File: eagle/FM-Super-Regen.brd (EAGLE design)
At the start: 41.9 x 21.6 mm, 15 parts, among them Q1 BF245B

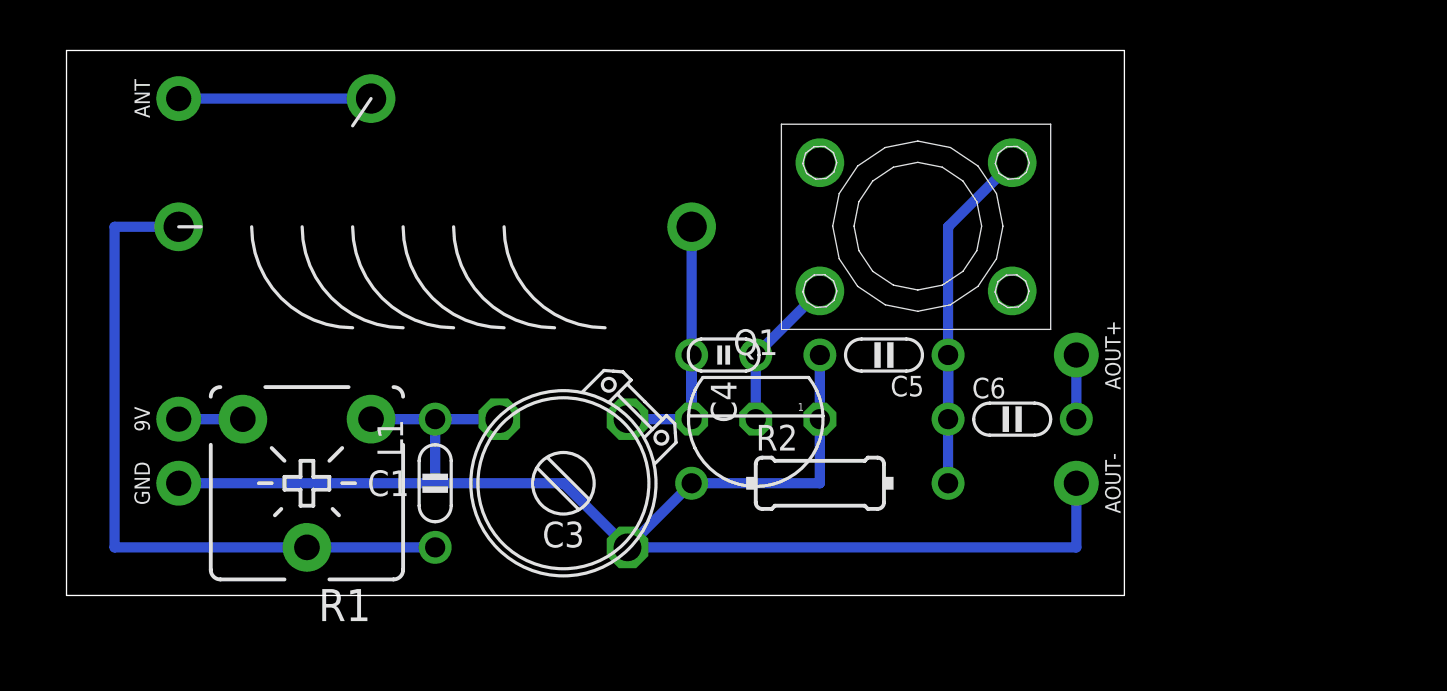
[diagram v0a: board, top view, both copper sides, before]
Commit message: ...
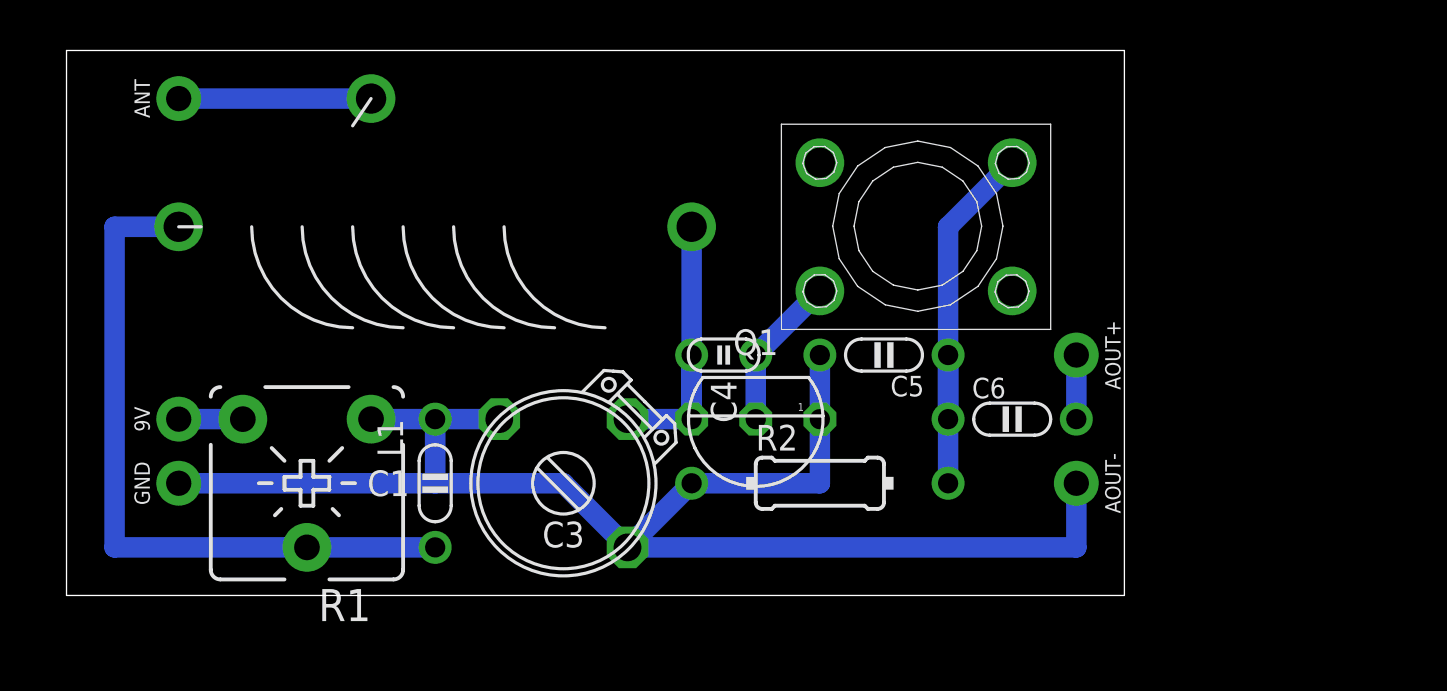
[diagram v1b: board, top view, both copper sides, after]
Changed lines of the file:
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@@
 <?xml version="1.0" encoding="utf-8"?>
 <!DOCTYPE eagle SYSTEM "eagle.dtd">
-<eagle version="7.7.0">
+<eagle version="7.6.0">
 <drawing>
 <settings>
@@
 <contactref element="AOUT-" pad="1"/>
 <contactref element="GND" pad="1"/>
-<wire x1="30.48" y1="7.62" x2="30.48" y2="5.08" width="0.4064" layer="16"/>
-<wire x1="12.7" y1="7.62" x2="15.24" y2="7.62" width="0.4064" layer="16"/>
-<wire x1="5.08" y1="5.08" x2="15.24" y2="5.08" width="0.4064" layer="16"/>
-<wire x1="15.24" y1="5.08" x2="20.32" y2="5.08" width="0.4064" layer="16"/>
-<wire x1="20.32" y1="5.08" x2="22.86" y2="2.54" width="0.4064" layer="16"/>
-<wire x1="17.78" y1="7.62" x2="15.24" y2="7.62" width="0.4064" layer="16"/>
-<wire x1="15.24" y1="7.62" x2="15.24" y2="5.08" width="0.4064" layer="16"/>
-<wire x1="40.64" y1="5.08" x2="40.64" y2="2.54" width="0.4064" layer="16"/>
-<wire x1="40.64" y1="2.54" x2="22.86" y2="2.54" width="0.4064" layer="16"/>
-<wire x1="22.86" y1="2.54" x2="25.4" y2="5.08" width="0.4064" layer="16"/>
-<wire x1="25.4" y1="5.08" x2="30.48" y2="5.08" width="0.4064" layer="16"/>
-<wire x1="30.48" y1="7.62" x2="30.48" y2="10.16" width="0.4064" layer="16"/>
+<wire x1="30.48" y1="7.62" x2="30.48" y2="5.08" width="0.8128" layer="16"/>
+<wire x1="12.7" y1="7.62" x2="15.24" y2="7.62" width="0.8128" layer="16"/>
+<wire x1="5.08" y1="5.08" x2="15.24" y2="5.08" width="0.8128" layer="16"/>
+<wire x1="15.24" y1="5.08" x2="20.32" y2="5.08" width="0.8128" layer="16"/>
+<wire x1="20.32" y1="5.08" x2="22.86" y2="2.54" width="0.8128" layer="16"/>
+<wire x1="17.78" y1="7.62" x2="15.24" y2="7.62" width="0.8128" layer="16"/>
+<wire x1="15.24" y1="7.62" x2="15.24" y2="5.08" width="0.8128" layer="16"/>
+<wire x1="40.64" y1="5.08" x2="40.64" y2="2.54" width="0.8128" layer="16"/>
+<wire x1="40.64" y1="2.54" x2="22.86" y2="2.54" width="0.8128" layer="16"/>
+<wire x1="22.86" y1="2.54" x2="25.4" y2="5.08" width="0.8128" layer="16"/>
+<wire x1="25.4" y1="5.08" x2="30.48" y2="5.08" width="0.8128" layer="16"/>
+<wire x1="30.48" y1="7.62" x2="30.48" y2="10.16" width="0.8128" layer="16"/>
 </signal>
 <signal name="N$2">
@@
 <contactref element="C4" pad="1"/>
 <contactref element="C3" pad="2"/>
-<wire x1="25.4" y1="15.24" x2="25.4" y2="7.62" width="0.4064" layer="16"/>
-<wire x1="25.4" y1="10.16" x2="25.4" y2="7.62" width="0.4064" layer="16"/>
-<wire x1="25.4" y1="7.62" x2="22.86" y2="7.62" width="0.4064" layer="16"/>
+<wire x1="25.4" y1="15.24" x2="25.4" y2="7.62" width="0.8128" layer="16"/>
+<wire x1="25.4" y1="10.16" x2="25.4" y2="7.62" width="0.8128" layer="16"/>
+<wire x1="25.4" y1="7.62" x2="22.86" y2="7.62" width="0.8128" layer="16"/>
 </signal>
 <signal name="N$3">
@@
 <contactref element="C1" pad="1"/>
 <contactref element="R1" pad="S"/>
-<wire x1="15.24" y1="2.54" x2="10.16" y2="2.54" width="0.4064" layer="16"/>
-<wire x1="10.16" y1="2.54" x2="2.54" y2="2.54" width="0.4064" layer="16"/>
-<wire x1="2.54" y1="2.54" x2="2.54" y2="15.24" width="0.4064" layer="16"/>
-<wire x1="2.54" y1="15.24" x2="5.08" y2="15.24" width="0.4064" layer="16"/>
+<wire x1="15.24" y1="2.54" x2="10.16" y2="2.54" width="0.8128" layer="16"/>
+<wire x1="10.16" y1="2.54" x2="2.54" y2="2.54" width="0.8128" layer="16"/>
+<wire x1="2.54" y1="2.54" x2="2.54" y2="15.24" width="0.8128" layer="16"/>
+<wire x1="2.54" y1="15.24" x2="5.08" y2="15.24" width="0.8128" layer="16"/>
 </signal>
 <signal name="N$4">
 <contactref element="L1" pad="T"/>
 <contactref element="ANT" pad="1"/>
-<wire x1="12.7" y1="20.32" x2="5.08" y2="20.32" width="0.4064" layer="16"/>
+<wire x1="12.7" y1="20.32" x2="5.08" y2="20.32" width="0.8128" layer="16"/>
 </signal>
 <signal name="N$5">
@@
 <contactref element="Q1" pad="2"/>
 <contactref element="L2" pad="3"/>
-<wire x1="30.48" y1="12.7" x2="27.94" y2="10.16" width="0.4064" layer="16"/>
-<wire x1="27.94" y1="7.62" x2="27.94" y2="10.16" width="0.4064" layer="16"/>
+<wire x1="30.48" y1="12.7" x2="27.94" y2="10.16" width="0.8128" layer="16"/>
+<wire x1="27.94" y1="7.62" x2="27.94" y2="10.16" width="0.8128" layer="16"/>
 </signal>
 <signal name="N$6">
@@
 <contactref element="C5" pad="1"/>
 <contactref element="C6" pad="1"/>
-<wire x1="35.56" y1="5.08" x2="35.56" y2="10.16" width="0.4064" layer="16"/>
-<wire x1="35.56" y1="7.62" x2="35.56" y2="10.16" width="0.4064" layer="16"/>
-<wire x1="35.56" y1="10.16" x2="35.56" y2="15.24" width="0.4064" layer="16"/>
-<wire x1="35.56" y1="15.24" x2="38.1" y2="17.78" width="0.4064" layer="16"/>
+<wire x1="35.56" y1="5.08" x2="35.56" y2="10.16" width="0.8128" layer="16"/>
+<wire x1="35.56" y1="7.62" x2="35.56" y2="10.16" width="0.8128" layer="16"/>
+<wire x1="35.56" y1="10.16" x2="35.56" y2="15.24" width="0.8128" layer="16"/>
+<wire x1="35.56" y1="15.24" x2="38.1" y2="17.78" width="0.8128" layer="16"/>
 </signal>
 <signal name="N$8">
 <contactref element="AOUT+" pad="1"/>
 <contactref element="C6" pad="2"/>
-<wire x1="40.64" y1="10.16" x2="40.64" y2="7.62" width="0.4064" layer="16"/>
+<wire x1="40.64" y1="10.16" x2="40.64" y2="7.62" width="0.8128" layer="16"/>
 </signal>
 <signal name="N$1">
 <contactref element="9V" pad="1"/>
 <contactref element="R1" pad="E"/>
-<wire x1="5.08" y1="7.62" x2="7.62" y2="7.62" width="0.4064" layer="16"/>
+<wire x1="5.08" y1="7.62" x2="7.62" y2="7.62" width="0.8128" layer="16"/>
 </signal>
 </signals>

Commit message: ...
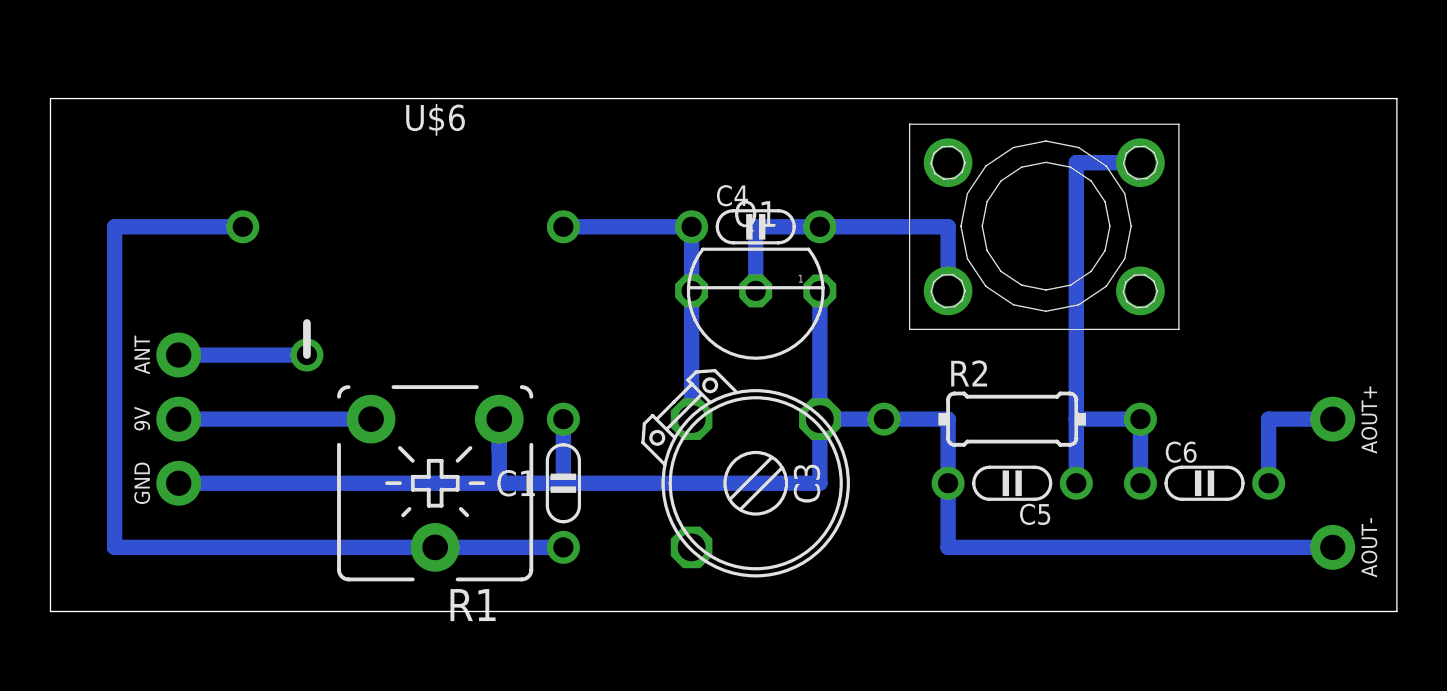
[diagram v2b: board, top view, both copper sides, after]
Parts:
- removed L1: 0.22uH, l:L-08/7V-TAP1
- added U$6: 0.22uH, l:L-08/10-TAP1
- C4: value 47p -> 4.7pF; device c:C025-015X024 -> c:C050-020X036
- moved AOUT+ 10.5 mm to (50.8, 7.62)
- moved AOUT- 10.5 mm to (50.8, 2.54)
- moved ANT 10.2 mm to (5.08, 10.2)
- moved R2 8.03 mm to (38.1, 7.62)
- moved C6 8.03 mm to (45.7, 5.08)
- moved C3 7.62 mm to (27.9, 5.08), turned to 270 degrees
- moved C5 7.18 mm to (38.1, 5.08)
- moved C4 5.24 mm to (27.9, 15.2), turned to 0 degrees
- moved C1 5.08 mm to (20.3, 5.08)
- moved R1 5.08 mm to (15.2, 5.08)
- moved Q1 5.08 mm to (27.9, 12.7)
- moved L2 5.08 mm to (39.4, 15.2)
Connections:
- net N$2: now also U$6.2; no longer L1.2
- net N$3: now also U$6.1; no longer L1.1
- net N$4: now also U$6.3; no longer L1.T
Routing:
- net N$3: track 27.9 -> 35.6 mm
- net N$5: track 6.13 -> 12.7 mm
- net N$1: track 2.54 -> 7.62 mm
- net GND: track 60.5 -> 64.8 mm
- net N$6: track 16.3 -> 20.3 mm
- net N$8: track 2.54 -> 5.08 mm
- net N$4: track 7.62 -> 5.08 mm
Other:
- board size 41.9 x 21.6 mm -> 53.3 x 20.3 mm
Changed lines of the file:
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@@
 http://ryanzachry.com/2013/01/super-regen-fm-radio/</description>
 <plain>
-<wire x1="0.635" y1="0.635" x2="42.545" y2="0.635" width="0" layer="20"/>
-<wire x1="42.545" y1="0.635" x2="42.545" y2="22.225" width="0" layer="20"/>
-<wire x1="42.545" y1="22.225" x2="0.635" y2="22.225" width="0" layer="20"/>
-<wire x1="0.635" y1="22.225" x2="0.635" y2="0.635" width="0" layer="20"/>
+<wire x1="0" y1="0" x2="53.34" y2="0" width="0" layer="20"/>
+<wire x1="53.34" y1="0" x2="53.34" y2="20.32" width="0" layer="20"/>
+<wire x1="53.34" y1="20.32" x2="0" y2="20.32" width="0" layer="20"/>
+<wire x1="0" y1="20.32" x2="0" y2="0" width="0" layer="20"/>
 </plain>
 <attributes>
@@
 <elements>
 <element name="9V" library="pad" package="SPAD" value="SPAD" x="5.08" y="7.62"/>
-<element name="ANT" library="pad" package="SPAD" value="ANT" x="5.08" y="20.32"/>
-<element name="AOUT+" library="pad" package="SPAD" value="SPAD" x="40.64" y="10.16" rot="R180"/>
-<element name="AOUT-" library="pad" package="SPAD" value="SPAD" x="40.64" y="5.08" rot="R180"/>
-<element name="C1" library="c" package="C050-020X036/V" value="1n" x="15.24" y="5.08"/>
-<element name="C3" library="cap-trim" package="TRIM-2222-808" value="15p" x="20.32" y="5.08" rot="R180"/>
-<element name="C4" library="c" package="C025-015X024" value="47p" x="26.67" y="10.16" rot="R90"/>
-<element name="C5" library="c" package="C050-020X036" value="4.7n" x="33.02" y="10.16" rot="R180"/>
-<element name="C6" library="c" package="C050-020X036" value="100n" x="38.1" y="7.62"/>
+<element name="ANT" library="pad" package="SPAD" value="ANT" x="5.08" y="10.16"/>
+<element name="AOUT+" library="pad" package="SPAD" value="SPAD" x="50.8" y="7.62" rot="R180"/>
+<element name="AOUT-" library="pad" package="SPAD" value="SPAD" x="50.8" y="2.54" rot="R180"/>
+<element name="C1" library="c" package="C050-020X036/V" value="1n" x="20.32" y="5.08" smashed="yes">
+<attribute name="NAME" x="19.304" y="5.08" size="1.016" layer="25" align="center-right"/>
+<attribute name="VALUE" x="20.066" y="1.27" size="1.016" layer="27" align="center-left"/>
+</element>
+<element name="C3" library="cap-trim" package="TRIM-2222-808" value="15p" x="27.94" y="5.08" rot="R270"/>
+<element name="C4" library="c" package="C050-020X036" value="4.7pF" x="27.94" y="15.24"/>
+<element name="C5" library="c" package="C050-020X036" value="4.7n" x="38.1" y="5.08" rot="R180"/>
+<element name="C6" library="c" package="C050-020X036" value="100n" x="45.72" y="5.08"/>
 <element name="GND" library="pad" package="SPAD" value="SPAD" x="5.08" y="5.08"/>
-<element name="L1" library="l" package="L-08/7V-TAP1" value="0.22uH" x="15.24" y="15.24" rot="R90"/>
-<element name="L2" library="l" package="L-BODY" value="3.3uH" x="34.29" y="15.24"/>
-<element name="Q1" library="t" package="TO92" value="BF245B" x="27.94" y="7.62" rot="R180"/>
-<element name="R1" library="r" package="POT-V" value="1k" x="10.16" y="5.08" rot="R180"/>
-<element name="R2" library="r" package="0204/10" value="10k" x="30.48" y="5.08"/>
+<element name="L2" library="l" package="L-BODY" value="3.3uH" x="39.37" y="15.24"/>
+<element name="Q1" library="t" package="TO92" value="BF245B" x="27.94" y="12.7" rot="R180"/>
+<element name="R1" library="r" package="POT-V" value="1k" x="15.24" y="5.08" rot="R180"/>
+<element name="R2" library="r" package="0204/10" value="10k" x="38.1" y="7.62"/>
+<element name="U$6" library="l" package="L-08/10-TAP1" value="0.22uH" x="13.97" y="15.24"/>
 </elements>
 <signals>
@@
 <contactref element="AOUT-" pad="1"/>
 <contactref element="GND" pad="1"/>
-<wire x1="30.48" y1="7.62" x2="30.48" y2="5.08" width="0.8128" layer="16"/>
-<wire x1="12.7" y1="7.62" x2="15.24" y2="7.62" width="0.8128" layer="16"/>
-<wire x1="5.08" y1="5.08" x2="15.24" y2="5.08" width="0.8128" layer="16"/>
-<wire x1="15.24" y1="5.08" x2="20.32" y2="5.08" width="0.8128" layer="16"/>
-<wire x1="20.32" y1="5.08" x2="22.86" y2="2.54" width="0.8128" layer="16"/>
-<wire x1="17.78" y1="7.62" x2="15.24" y2="7.62" width="0.8128" layer="16"/>
-<wire x1="15.24" y1="7.62" x2="15.24" y2="5.08" width="0.8128" layer="16"/>
-<wire x1="40.64" y1="5.08" x2="40.64" y2="2.54" width="0.8128" layer="16"/>
-<wire x1="40.64" y1="2.54" x2="22.86" y2="2.54" width="0.8128" layer="16"/>
-<wire x1="22.86" y1="2.54" x2="25.4" y2="5.08" width="0.8128" layer="16"/>
-<wire x1="25.4" y1="5.08" x2="30.48" y2="5.08" width="0.8128" layer="16"/>
-<wire x1="30.48" y1="7.62" x2="30.48" y2="10.16" width="0.8128" layer="16"/>
+<wire x1="30.48" y1="5.08" x2="20.32" y2="5.08" width="0.6096" layer="16"/>
+<wire x1="17.78" y1="7.62" x2="17.78" y2="6.35" width="0.6096" layer="16"/>
+<wire x1="17.78" y1="5.08" x2="5.08" y2="5.08" width="0.6096" layer="16"/>
+<wire x1="30.48" y1="5.08" x2="30.48" y2="7.62" width="0.6096" layer="16"/>
+<wire x1="50.8" y1="2.54" x2="35.56" y2="2.54" width="0.6096" layer="16"/>
+<wire x1="35.56" y1="2.54" x2="35.56" y2="5.08" width="0.6096" layer="16"/>
+<wire x1="33.02" y1="7.62" x2="35.56" y2="7.62" width="0.6096" layer="16"/>
+<wire x1="35.56" y1="7.62" x2="35.56" y2="5.08" width="0.6096" layer="16"/>
+<wire x1="30.48" y1="12.7" x2="30.48" y2="7.62" width="0.6096" layer="16"/>
+<wire x1="30.48" y1="7.62" x2="33.02" y2="7.62" width="0.6096" layer="16"/>
+<wire x1="17.78" y1="7.62" x2="17.78" y2="5.08" width="0.6096" layer="16"/>
+<wire x1="17.78" y1="5.08" x2="20.32" y2="5.08" width="0.6096" layer="16"/>
+<wire x1="20.32" y1="5.08" x2="20.32" y2="7.62" width="0.6096" layer="16"/>
 </signal>
 <signal name="N$2">
 <contactref element="Q1" pad="3"/>
-<contactref element="L1" pad="2"/>
 <contactref element="C4" pad="1"/>
 <contactref element="C3" pad="2"/>
-<wire x1="25.4" y1="15.24" x2="25.4" y2="7.62" width="0.8128" layer="16"/>
-<wire x1="25.4" y1="10.16" x2="25.4" y2="7.62" width="0.8128" layer="16"/>
-<wire x1="25.4" y1="7.62" x2="22.86" y2="7.62" width="0.8128" layer="16"/>
+<wire x1="25.4" y1="7.62" x2="25.4" y2="12.7" width="0.6096" layer="16"/>
+<wire x1="25.4" y1="12.7" x2="25.4" y2="15.24" width="0.6096" layer="16"/>
+<contactref element="U$6" pad="2"/>
+<wire x1="20.32" y1="15.24" x2="25.4" y2="15.24" width="0.6096" layer="16"/>
 </signal>
 <signal name="N$3">
-<contactref element="L1" pad="1"/>
 <contactref element="C1" pad="1"/>
 <contactref element="R1" pad="S"/>
-<wire x1="15.24" y1="2.54" x2="10.16" y2="2.54" width="0.8128" layer="16"/>
-<wire x1="10.16" y1="2.54" x2="2.54" y2="2.54" width="0.8128" layer="16"/>
-<wire x1="2.54" y1="2.54" x2="2.54" y2="15.24" width="0.8128" layer="16"/>
-<wire x1="2.54" y1="15.24" x2="5.08" y2="15.24" width="0.8128" layer="16"/>
+<wire x1="20.32" y1="2.54" x2="15.24" y2="2.54" width="0.6096" layer="16"/>
+<wire x1="15.24" y1="2.54" x2="2.54" y2="2.54" width="0.6096" layer="16"/>
+<contactref element="U$6" pad="1"/>
+<wire x1="2.54" y1="2.54" x2="2.54" y2="15.24" width="0.6096" layer="16"/>
+<wire x1="2.54" y1="15.24" x2="7.62" y2="15.24" width="0.6096" layer="16"/>
 </signal>
 <signal name="N$4">
-<contactref element="L1" pad="T"/>
 <contactref element="ANT" pad="1"/>
-<wire x1="12.7" y1="20.32" x2="5.08" y2="20.32" width="0.8128" layer="16"/>
+<contactref element="U$6" pad="3"/>
+<wire x1="5.08" y1="10.16" x2="10.16" y2="10.16" width="0.6096" layer="16"/>
 </signal>
 <signal name="N$5">
@@
 <contactref element="Q1" pad="2"/>
 <contactref element="L2" pad="3"/>
-<wire x1="30.48" y1="12.7" x2="27.94" y2="10.16" width="0.8128" layer="16"/>
-<wire x1="27.94" y1="7.62" x2="27.94" y2="10.16" width="0.8128" layer="16"/>
+<wire x1="27.94" y1="12.7" x2="27.94" y2="15.24" width="0.6096" layer="16"/>
+<wire x1="27.94" y1="15.24" x2="30.48" y2="15.24" width="0.6096" layer="16"/>
+<wire x1="30.48" y1="15.24" x2="35.56" y2="15.24" width="0.6096" layer="16"/>
+<wire x1="35.56" y1="15.24" x2="35.56" y2="12.7" width="0.6096" layer="16"/>
 </signal>
 <signal name="N$6">
@@
 <contactref element="C5" pad="1"/>
 <contactref element="C6" pad="1"/>
-<wire x1="35.56" y1="5.08" x2="35.56" y2="10.16" width="0.8128" layer="16"/>
-<wire x1="35.56" y1="7.62" x2="35.56" y2="10.16" width="0.8128" layer="16"/>
-<wire x1="35.56" y1="10.16" x2="35.56" y2="15.24" width="0.8128" layer="16"/>
-<wire x1="35.56" y1="15.24" x2="38.1" y2="17.78" width="0.8128" layer="16"/>
+<wire x1="43.18" y1="17.78" x2="40.64" y2="17.78" width="0.6096" layer="16"/>
+<wire x1="40.64" y1="17.78" x2="40.64" y2="7.62" width="0.6096" layer="16"/>
+<wire x1="40.64" y1="5.08" x2="40.64" y2="7.62" width="0.6096" layer="16"/>
+<wire x1="40.64" y1="7.62" x2="43.18" y2="7.62" width="0.6096" layer="16"/>
+<wire x1="43.18" y1="5.08" x2="43.18" y2="7.62" width="0.6096" layer="16"/>
 </signal>
 <signal name="N$8">
 <contactref element="AOUT+" pad="1"/>
 <contactref element="C6" pad="2"/>
-<wire x1="40.64" y1="10.16" x2="40.64" y2="7.62" width="0.8128" layer="16"/>
+<wire x1="48.26" y1="5.08" x2="48.26" y2="7.62" width="0.6096" layer="16"/>
+<wire x1="48.26" y1="7.62" x2="50.8" y2="7.62" width="0.6096" layer="16"/>
 </signal>
 <signal name="N$1">
 <contactref element="9V" pad="1"/>
 <contactref element="R1" pad="E"/>
-<wire x1="5.08" y1="7.62" x2="7.62" y2="7.62" width="0.8128" layer="16"/>
+<wire x1="5.08" y1="7.62" x2="12.7" y2="7.62" width="0.6096" layer="16"/>
 </signal>
 </signals>
